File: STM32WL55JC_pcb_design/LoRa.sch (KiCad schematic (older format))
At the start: 22 parts, among them IC2 PE4259, J16 Conn_Coaxial

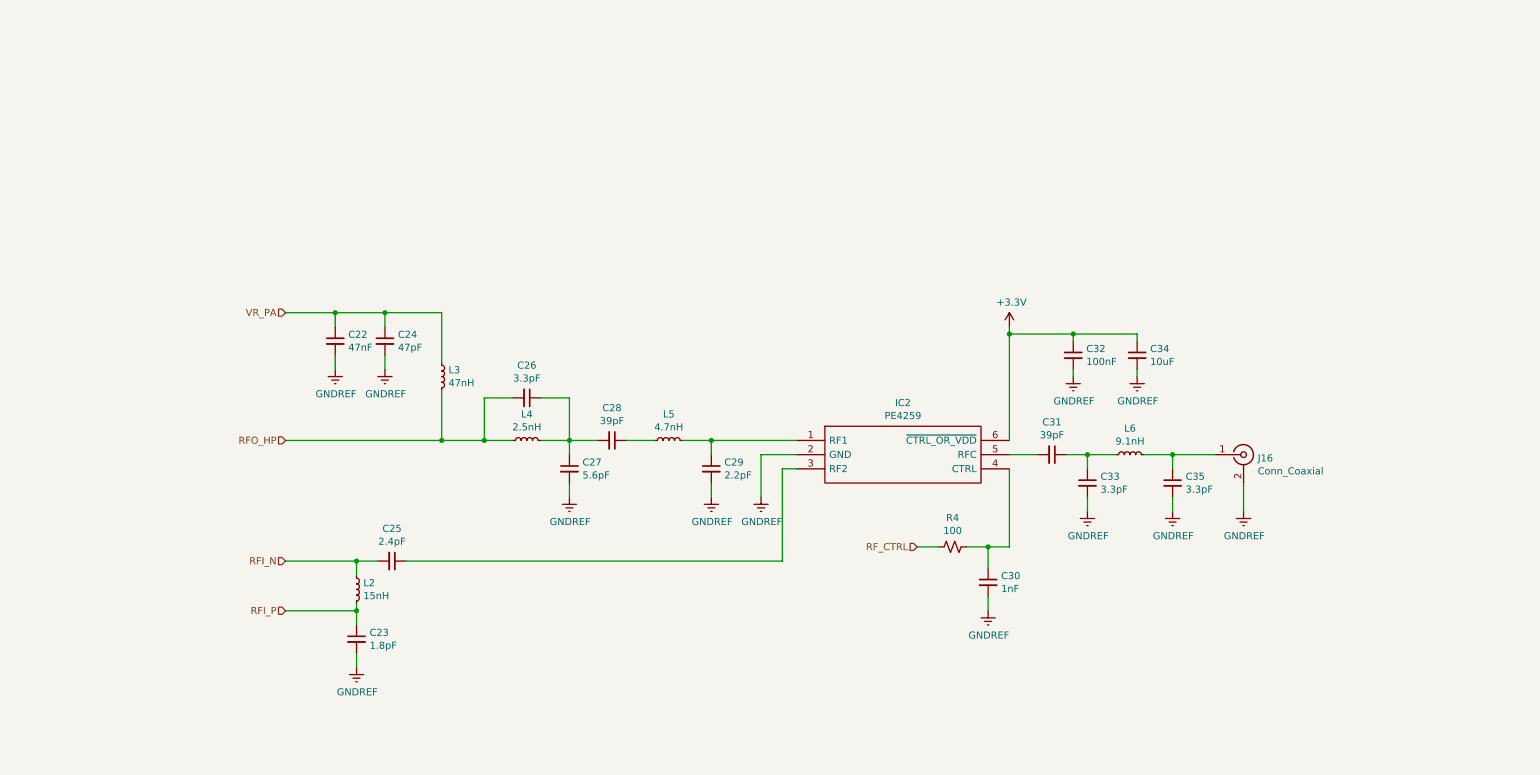
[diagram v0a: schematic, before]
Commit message: Finish new design schematic
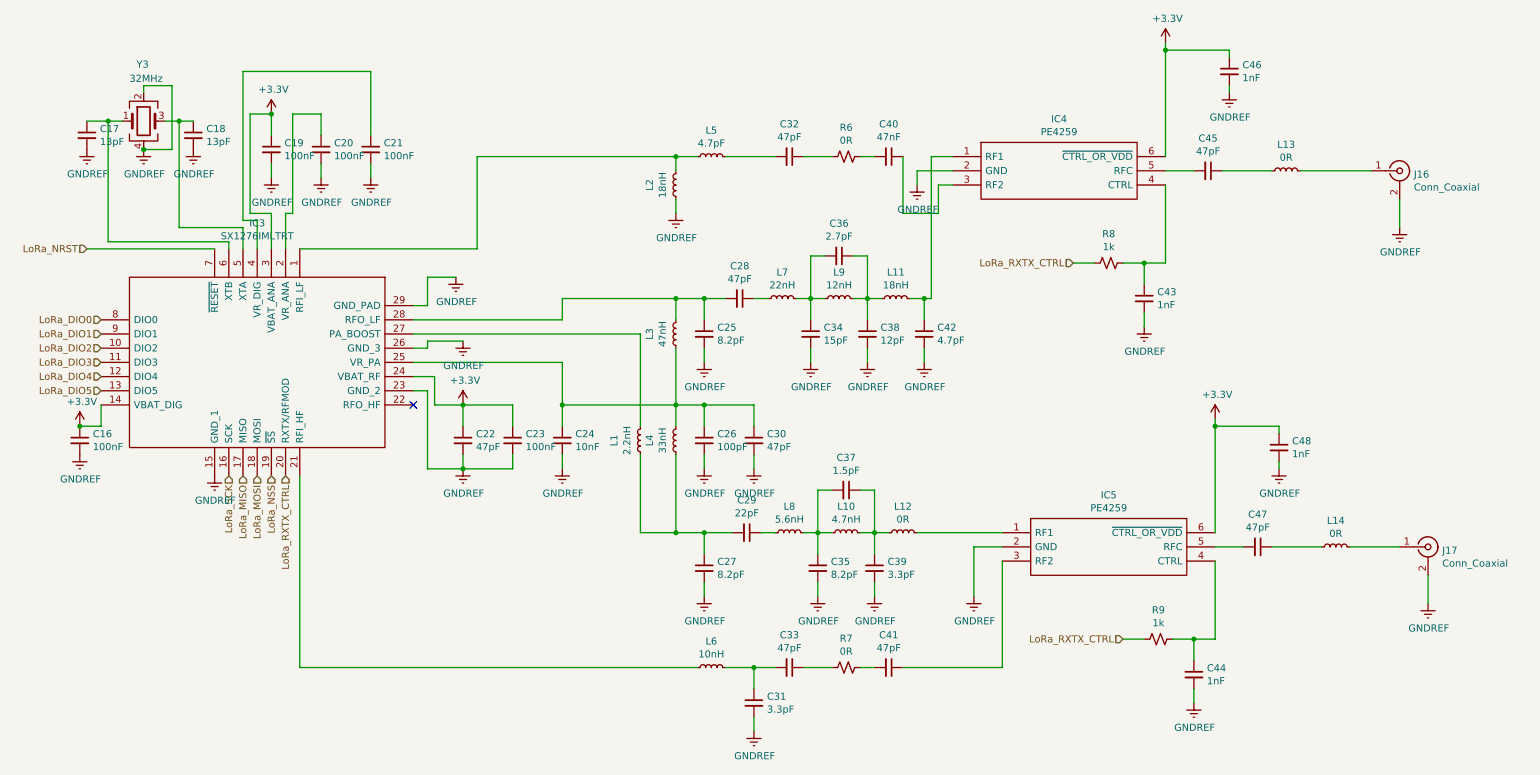
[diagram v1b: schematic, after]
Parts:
- removed L5: 4.7nH, Inductor_SMD:L_0805_2012Metric, symbol Device:L_Small
- added C16, C19, C20, C21, C23: 100nF, Capacitor_SMD:C_0805_2012Metric, symbol Device:C_Small
- added C17, C18: 13pF, Capacitor_SMD:C_0805_2012Metric, symbol Device:C_Small
- added C30, C41, C47: 47pF, Capacitor_SMD:C_0805_2012Metric, symbol Device:C_Small
- added C31, C39: 3.3pF, Capacitor_SMD:C_0805_2012Metric, symbol Device:C_Small
- added C36: 2.7pF, Capacitor_SMD:C_0603_1608Metric, symbol Device:C_Small
- added C37: 1.5pF, Capacitor_SMD:C_0603_1608Metric, symbol Device:C_Small
- added C38: 12pF, Capacitor_SMD:C_0805_2012Metric, symbol Device:C_Small
- added C40: 47nF, Capacitor_SMD:C_0805_2012Metric, symbol Device:C_Small
- added C42: 4.7pF, Capacitor_SMD:C_0805_2012Metric, symbol Device:C_Small
- added C44, C48: 1nF, Capacitor_SMD:C_0805_2012Metric, symbol Device:C_Small
- added IC3: SX1276IMLTRT, QFN65P600X600X100-29N, symbol SX1276IMLTRT:SX1276IMLTRT
- added IC5: PE4259, PE4259:SOT65P210X110-6N, symbol PE4259:PE4259
- added J17: Conn_Coaxial, Connector_Coaxial:SMA_Amphenol_901-144_Vertical, symbol Connector:Conn_Coaxial
- added L1: 2.2nH, Inductor_SMD:L_0402_1005Metric, symbol Device:L_Small
- added L10: 4.7nH, Inductor_SMD:L_0402_1005Metric, symbol Device:L_Small
- added L11: 18nH, Inductor_SMD:L_0402_1005Metric, symbol Device:L_Small
- added L12, L14: 0R, Inductor_SMD:L_0402_1005Metric, symbol Device:L_Small
- added L4: 33nH, Inductor_SMD:L_0402_1005Metric, symbol Device:L_Small
- added L6: 10nH, Inductor_SMD:L_0402_1005Metric, symbol Device:L_Small
- added L7: 22nH, Inductor_SMD:L_0402_1005Metric, symbol Device:L_Small
- added L8: 5.6nH, Inductor_SMD:L_0402_1005Metric, symbol Device:L_Small
- added L9: 12nH, Inductor_SMD:L_0402_1005Metric, symbol Device:L_Small
- added R6, R7: 0R, Resistor_SMD:R_0805_2012Metric, symbol Device:R_Small_US
- added R9: 1k, Resistor_SMD:R_0805_2012Metric, symbol Device:R_Small_US
- added Y3: 32MHz, NX2016SA32MEXS00ACS06465:NX2016SA32MEXS00ACS06465, symbol Device:Crystal_GND24
- C22: value 47nF -> 47pF
- C24: value 47pF -> 10nF
- C25: renamed from C23; value 1.8pF -> 8.2pF
- C26: value 3.3pF -> 100pF
- C27: value 5.6pF -> 8.2pF
- C28: renamed from C25; value 2.4pF -> 47pF
- C29: value 2.2pF -> 22pF; footprint Capacitor_SMD:C_0402_1005Metric -> Capacitor_SMD:C_0805_2012Metric
- C32: renamed from C28; value 39pF -> 47pF
- C33: value 3.3pF -> 47pF
- C34: value 10uF -> 15pF
- C35: value 3.3pF -> 8.2pF
- C45: renamed from C31; value 39pF -> 47pF
- C46: renamed from C32; value 100nF -> 1nF
- L13: renamed from L6; value 9.1nH -> 0R
- L2: value 15nH -> 18nH; footprint Inductor_SMD:L_01005_0402Metric -> Inductor_SMD:L_0402_1005Metric
- L3: footprint Inductor_SMD:L_0805_2012Metric -> Inductor_SMD:L_0402_1005Metric
- L5: renamed from L4; value 2.5nH -> 4.7pF
- R8: renamed from R4; value 100 -> 1k
- renumbered C30 to C43, IC2 to IC4
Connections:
- net +3V3: now also C22.1, C16.1, C19.1, C23.1, C48.1, IC3.14 (VBAT_DIG), IC3.24 (VBAT_RF), IC3.3 (VBAT_ANA), IC5.6 (~CTRL_OR_VDD); no longer C34.1
- net GNDREF: now also C26.2, L2.1, C16.2, C17.2, C18.2, C19.2, C20.2, C21.2, C23.2, C30.2, C31.2, C38.2, C39.2, C42.2, C44.2, C48.2, IC3.15 (GND_1), IC3.23 (GND_2), IC3.26 (GND_3), IC3.29 (GND_PAD), IC5.2 (GND), J17.2 (Ext), Y3.2, Y3.4; no longer C29.2, C33.2
- net at J16.1 (In), L13.2: no longer C35.1
- net at C32.2, L5.2: no longer C26.1, C27.1
- net at C32.1: now also R6.1
- net at IC4.1 (RF1): now also C42.1, L11.2; no longer C29.1
- net at C28.1: now also L7.1; no longer IC4.3 (RF2)
- net at C45.1, L13.1: no longer C33.1
- net RFI_N: no longer names the net of C28.2
- net RFI_N: now also C25.1, L3.2, IC3.28 (RFO_LF); no longer L2.1
- net RFI_P: no longer names the net of L2.2
- net RFI_P: now also L5.1, IC3.1 (RFI_LF); no longer C25.1
- removed net RFO_HP: C26.2, L3.2, L5.1
- net RF_CTRL renamed LoRa_RXTX_CTRL
- net LoRa_RXTX_CTRL: now also IC3.20 (RXTX/RFMOD), R9.1
- net VR_PA: no longer names the net of C24.1, L3.1
- net VR_PA: now also C26.1, C30.1, IC3.25 (VR_PA), L4.2; no longer C22.1
- new net: C40.1, IC4.3 (RF2)
- new net: C27.1, C29.2, L1.1, L4.1
- new net: C29.1, L8.1
- new net: C35.1, C37.2, L10.1, L8.2
- new net: C37.1, C39.1, L10.2, L12.1
- new net: IC5.1 (RF1), L12.2
- new net: J17.1 (In), L14.2
- new net: C47.1, L14.1
- new net: C47.2, IC5.5 (RFC)
- new net: C41.1, IC5.3 (RF2)
- new net: C44.1, IC5.4 (CTRL), R9.2
- new net: C33.1, R7.1
- new net: C31.1, C33.2, L6.2
- new net: C41.2, R7.2
- new net: IC3.21 (RFI_HF), L6.1
- new net: C21.1, IC3.4 (VR_DIG)
- new net: C20.1, IC3.2 (VR_ANA)
- new net: C17.1, IC3.6 (XTB), Y3.1
- new net: C18.1, IC3.5 (XTA), Y3.3
- new net: C40.2, R6.2
- new net: C34.1, C36.2, L7.2, L9.1
- new net: C36.1, C38.1, L11.1, L9.2
- new net: IC3.27 (PA_BOOST), L1.2
- new net LoRa_DIO0: IC3.8 (DIO0)
- new net LoRa_DIO1: IC3.9 (DIO1)
- new net LoRa_DIO2: IC3.10 (DIO2)
- new net LoRa_DIO3: IC3.11 (DIO3)
- new net LoRa_DIO4: IC3.12 (DIO4)
- new net LoRa_DIO5: IC3.13 (DIO5)
- new net LoRa_MISO: IC3.17 (MISO)
- new net LoRa_MOSI: IC3.18 (MOSI)
- new net LoRa_NRST: IC3.7 (~RESET)
- new net LoRa_NSS: IC3.19 (~SS)
- new net LoRa_SCK: IC3.16 (SCK)
- no-connect marks 0 -> 1
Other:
- moved on the sheet: C25, C28, C32, C43, C45, C46, IC4, J16, L13, L5, R8
